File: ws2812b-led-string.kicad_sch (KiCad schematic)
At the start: 1 part

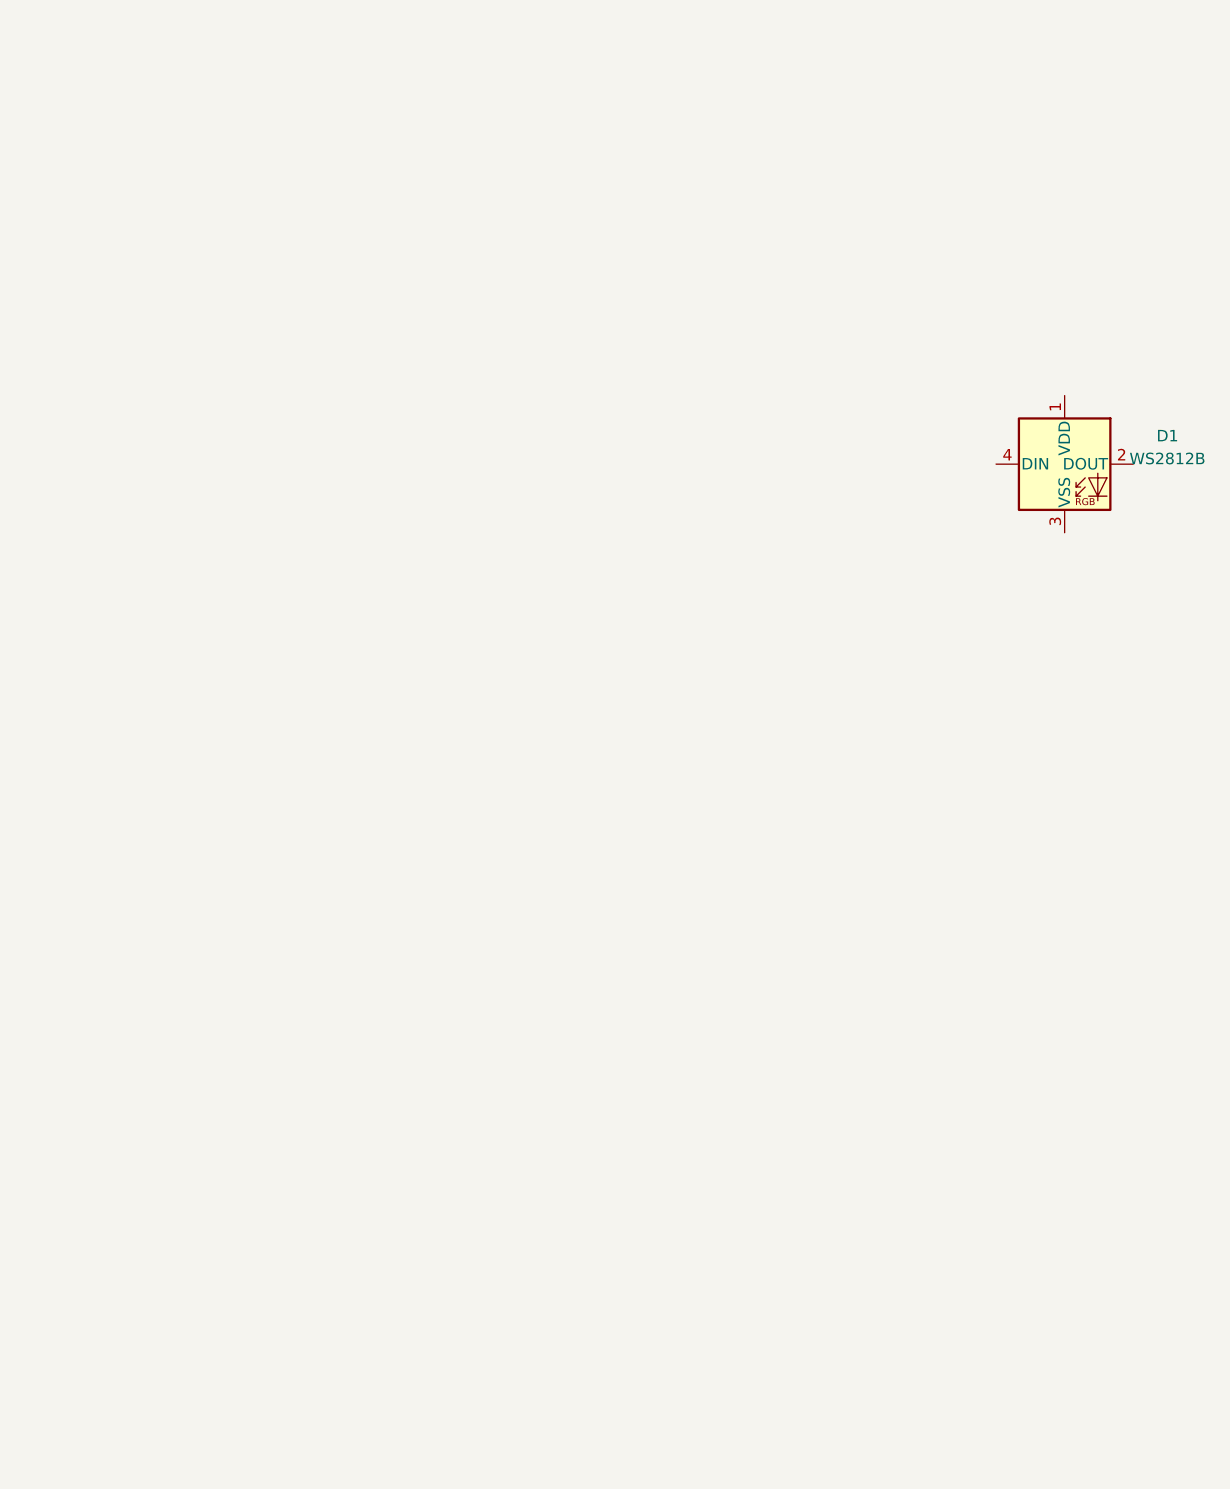
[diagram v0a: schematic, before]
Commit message: sdfdsfvsd
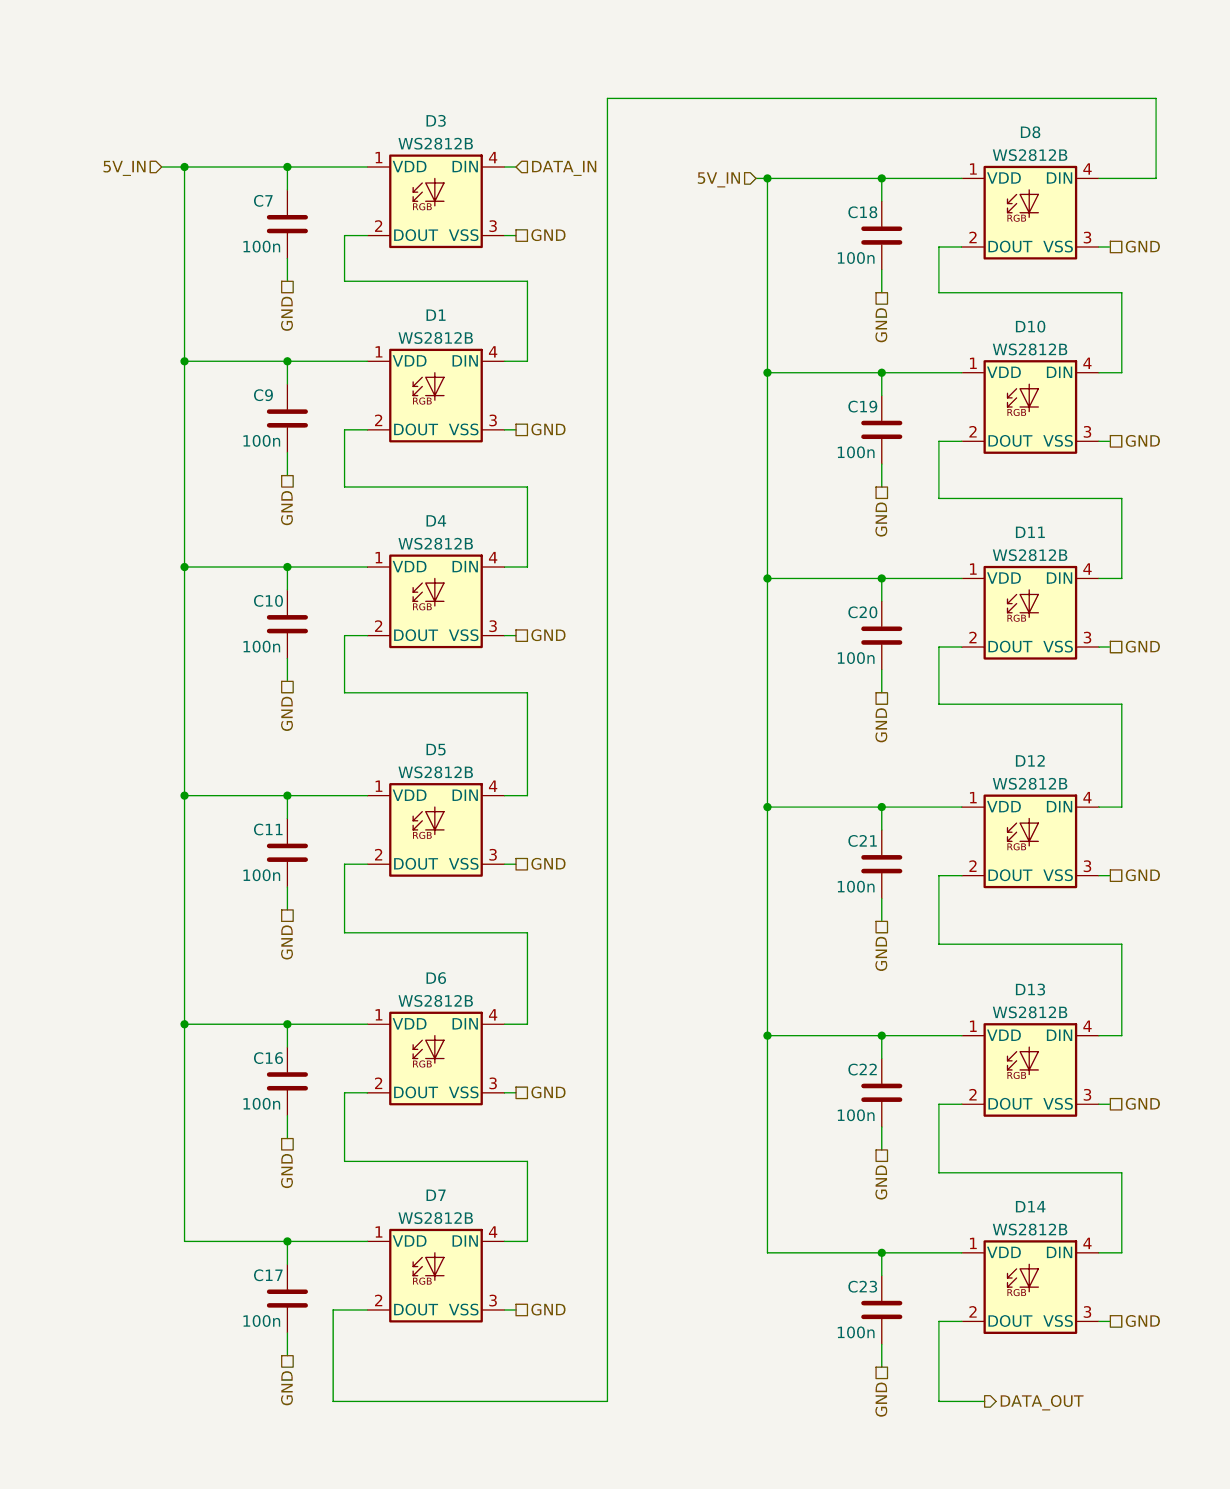
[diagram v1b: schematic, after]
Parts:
- removed D1: WS2812B, LED_SMD:LED_WS2812B_PLCC4_5.0x5.0mm_P3.2mm, symbol LED:WS2812B
- added C10, C11, C16, C17, C18, C19, C20, C21, C22, C23, C7, C9: 100n, Capacitor_SMD:C_0805_2012Metric_Pad1.18x1.45mm_HandSolder, symbol 000_Capacitor_Film_Immo:cap_film_0805
- added D1, D10, D11, D12, D13, D14, D3, D4, D5, D6, D7, D8: WS2812B, LED_SMD:LED_WS2812B_PLCC4_5.0x5.0mm_P3.2mm, symbol 000_Diodes_Immo:WS2812B
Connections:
- new net: D1.2 (DOUT), D4.4 (DIN)
- new net: D1.4 (DIN), D3.2 (DOUT)
- new net: D4.2 (DOUT), D5.4 (DIN)
- new net: D10.4 (DIN), D8.2 (DOUT)
- new net: D7.2 (DOUT), D8.4 (DIN)
- new net: D13.2 (DOUT), D14.4 (DIN)
- new net: D6.2 (DOUT), D7.4 (DIN)
- new net: D5.2 (DOUT), D6.4 (DIN)
- new net: D11.2 (DOUT), D12.4 (DIN)
- new net: D10.2 (DOUT), D11.4 (DIN)
- new net: D12.2 (DOUT), D13.4 (DIN)
- new net 5V_IN: C10.1, C11.1, C16.1, C17.1, C18.1, C19.1, C20.1, C21.1, C22.1, C23.1, C7.1, C9.1, D1.1 (VDD), D10.1 (VDD), D11.1 (VDD), D12.1 (VDD), D13.1 (VDD), D14.1 (VDD), D3.1 (VDD), D4.1 (VDD), D5.1 (VDD), D6.1 (VDD), D7.1 (VDD), D8.1 (VDD)
- new net DATA_IN: D3.4 (DIN)
- new net DATA_OUT: D14.2 (DOUT)
- new net GND: C10.2, C11.2, C16.2, C17.2, C18.2, C19.2, C20.2, C21.2, C22.2, C23.2, C7.2, C9.2, D1.3 (VSS), D10.3 (VSS), D11.3 (VSS), D12.3 (VSS), D13.3 (VSS), D14.3 (VSS), D3.3 (VSS), D4.3 (VSS), D5.3 (VSS), D6.3 (VSS), D7.3 (VSS), D8.3 (VSS)

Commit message: kjsaofklihsdof
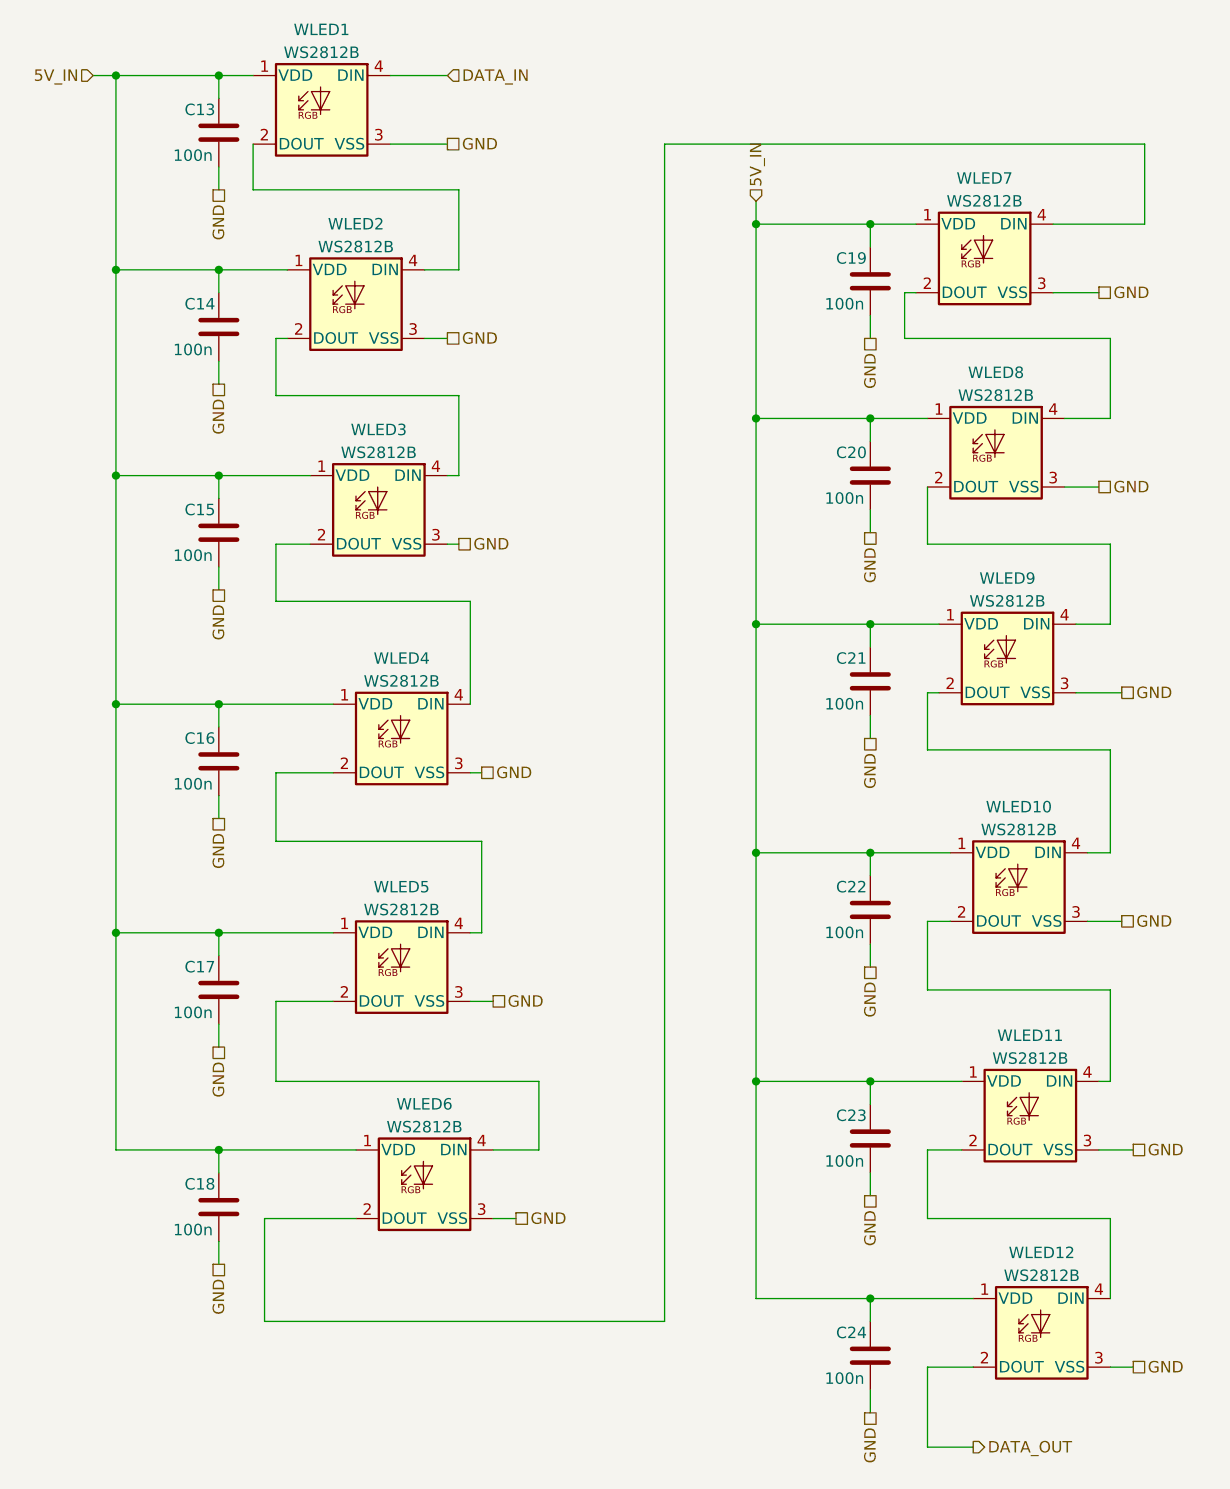
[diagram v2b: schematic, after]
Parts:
- renumbered C7 to C13, C9 to C14, C10 to C15, C11 to C16, C16 to C17, C17 to C18, C18 to C19, C19 to C20, C20 to C21, C21 to C22, C22 to C23, C23 to C24, D3 to WLED1, D12 to WLED10, D13 to WLED11, D14 to WLED12, D1 to WLED2, D4 to WLED3, D5 to WLED4, D6 to WLED5, D7 to WLED6, D8 to WLED7, D10 to WLED8, D11 to WLED9
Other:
- moved on the sheet: C13, C14, C15, C16, C17, C18, C19, C20, C21, C22, C23, C24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
